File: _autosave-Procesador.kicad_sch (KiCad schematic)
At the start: 62 parts, among them CN1 10way 1.27mm, J8 Micro_SD_Card_Det1, J9 RJ45_Wuerth_7499010211A, SW1 Reset, U20 24AA02E-OT, U21 FT900Q, U22 MCP9700Ax-ETT, Y1 Crystal, Y2 Crystal

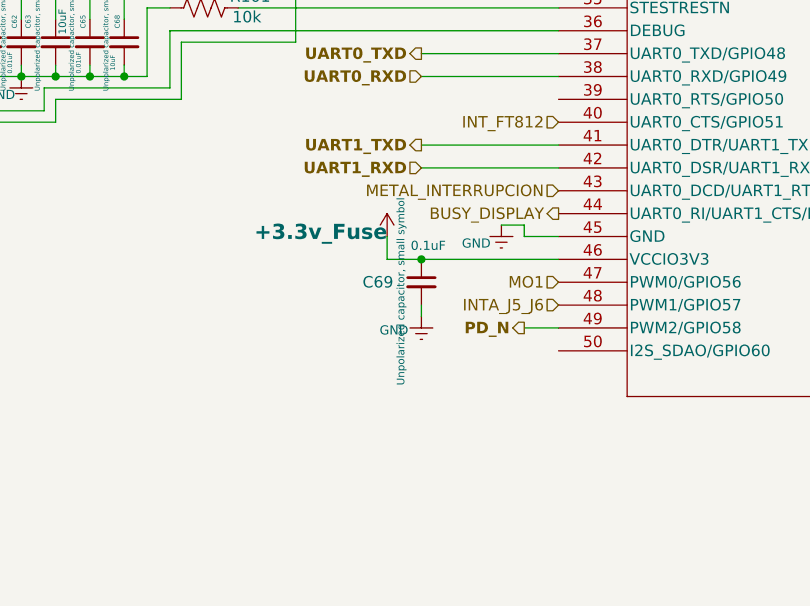
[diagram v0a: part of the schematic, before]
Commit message: 24/07/2026
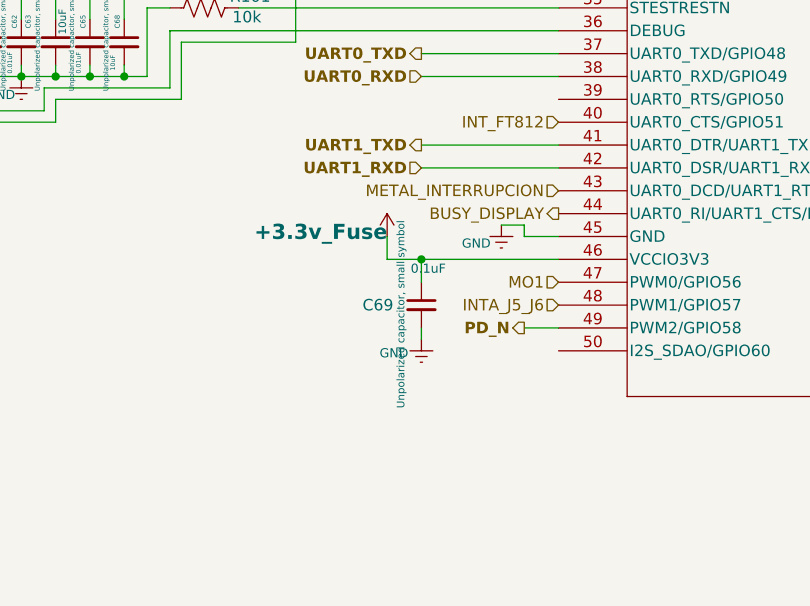
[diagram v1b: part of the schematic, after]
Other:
- moved on the sheet: C69
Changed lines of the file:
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@@
 	(wire
 		(pts
+			(xy 91.44 139.7) (xy 91.44 137.16)
+		)
+		(stroke
+			(width 0)
+			(type default)
+		)
+	)
+	(wire
+		(pts
 			(xy 256.54 62.23) (xy 256.54 68.58)
 		)
@@
 	(wire
 		(pts
-			(xy 91.44 142.24) (xy 91.44 143.51)
+			(xy 91.44 144.78) (xy 91.44 146.05)
 		)
 		(stroke
@@
 	(symbol
 		(lib_id "Device:C_Small")
-		(at 91.44 139.7 0)
+		(at 91.44 142.24 0)
 		(unit 1)
 		(exclude_from_sim no)
@@
 		(dnp no)
 		(property "Reference" "C69"
-			(at 86.614 139.7 0)
+			(at 86.614 142.24 0)
 			(effects
 				(font
@@
 		)
 		(property "Value" "0.1uF"
-			(at 92.202 135.636 0)
+			(at 92.202 138.176 0)
 			(effects
 				(font
@@
 		)
 		(property "Footprint" "Capacitor_SMD:C_0603_1608Metric_Pad1.08x0.95mm_HandSolder"
-			(at 91.44 139.7 0)
+			(at 91.44 142.24 0)
 			(effects
 				(font
@@
 		)
 		(property "Datasheet" "~"
-			(at 91.44 139.7 0)
+			(at 91.44 142.24 0)
 			(effects
 				(font
@@
 		)
 		(property "Description" "Unpolarized capacitor, small symbol"
-			(at 89.154 140.716 90)
+			(at 89.154 143.256 90)
 			(effects
 				(font
@@
 	(symbol
 		(lib_id "power:GNDREF")
-		(at 91.44 143.51 0)
+		(at 91.44 146.05 0)
 		(unit 1)
 		(exclude_from_sim no)
@@
 		(dnp no)
 		(property "Reference" "#PWR0304"
-			(at 91.44 149.86 0)
+			(at 91.44 152.4 0)
 			(effects
 				(font
@@
 		)
 		(property "Value" "GND"
-			(at 88.392 145.034 0)
+			(at 88.392 147.574 0)
 			(effects
 				(font
@@
 		)
 		(property "Footprint" ""
-			(at 91.44 143.51 0)
+			(at 91.44 146.05 0)
 			(effects
 				(font
@@
 		)
 		(property "Datasheet" ""
-			(at 91.44 143.51 0)
+			(at 91.44 146.05 0)
 			(effects
 				(font
@@
 		)
 		(property "Description" "Power symbol creates a global label with name \"GNDREF\" , reference supply ground"
-			(at 91.44 143.51 0)
+			(at 91.44 146.05 0)
 			(effects
 				(font
